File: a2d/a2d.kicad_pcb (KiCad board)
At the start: 4 copper layers, 70 x 65.8 mm, 76 parts, among them CN1 BM04B-SRSS-TB(LF)(SN), CN2 BM04B-SRSS-TB(LF)(SN), J1 Conn_02x04_Odd_Even, U1 B3B-XH-A(LF)(SN), U10 B3B-XH-A(LF)(SN), U2 2060-453/998-404, U3 ADM7150ARDZ-5.0, U4 ADS1115IDGSR, U5 2060-453/998-404, U6 B3B-XH-A(LF)(SN), U7 2060-453/998-404, U8 B3B-XH-A(LF)(SN), U9 2060-453/998-404

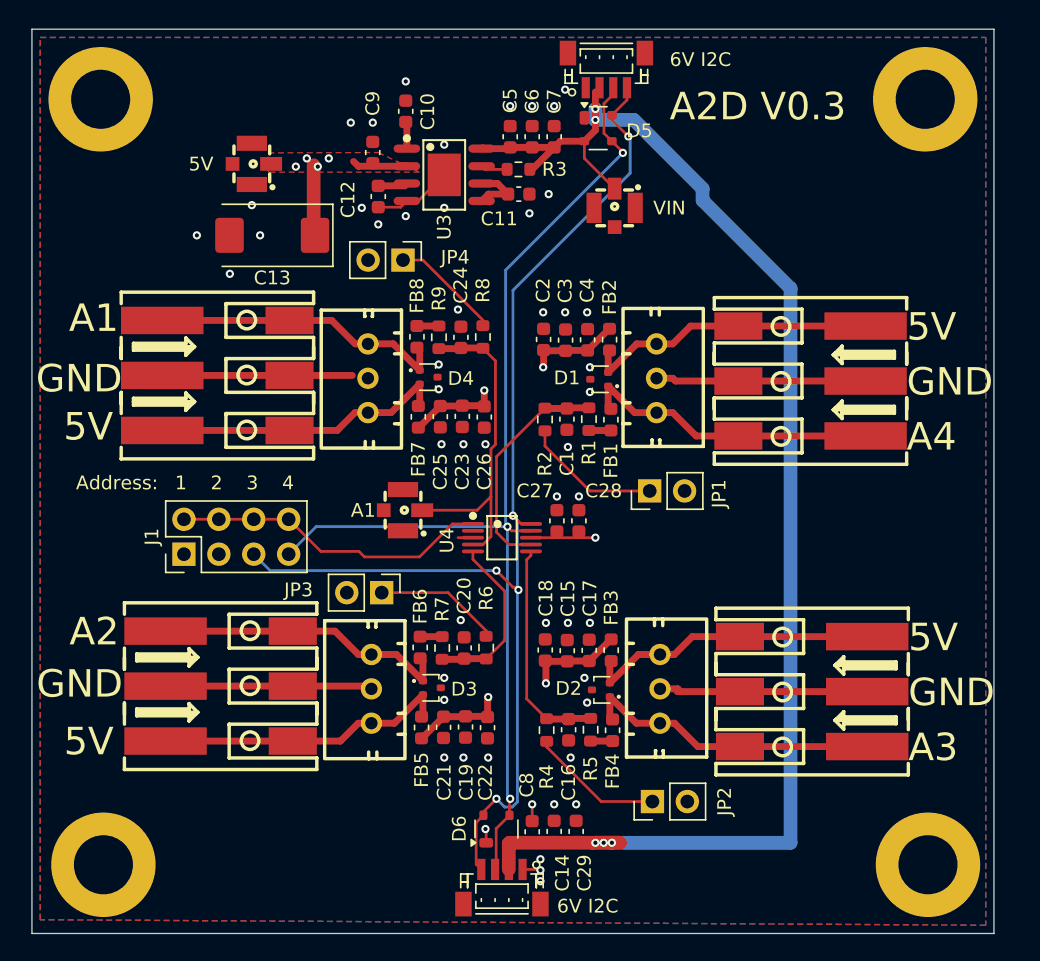
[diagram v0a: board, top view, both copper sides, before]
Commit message: a2d v0.4
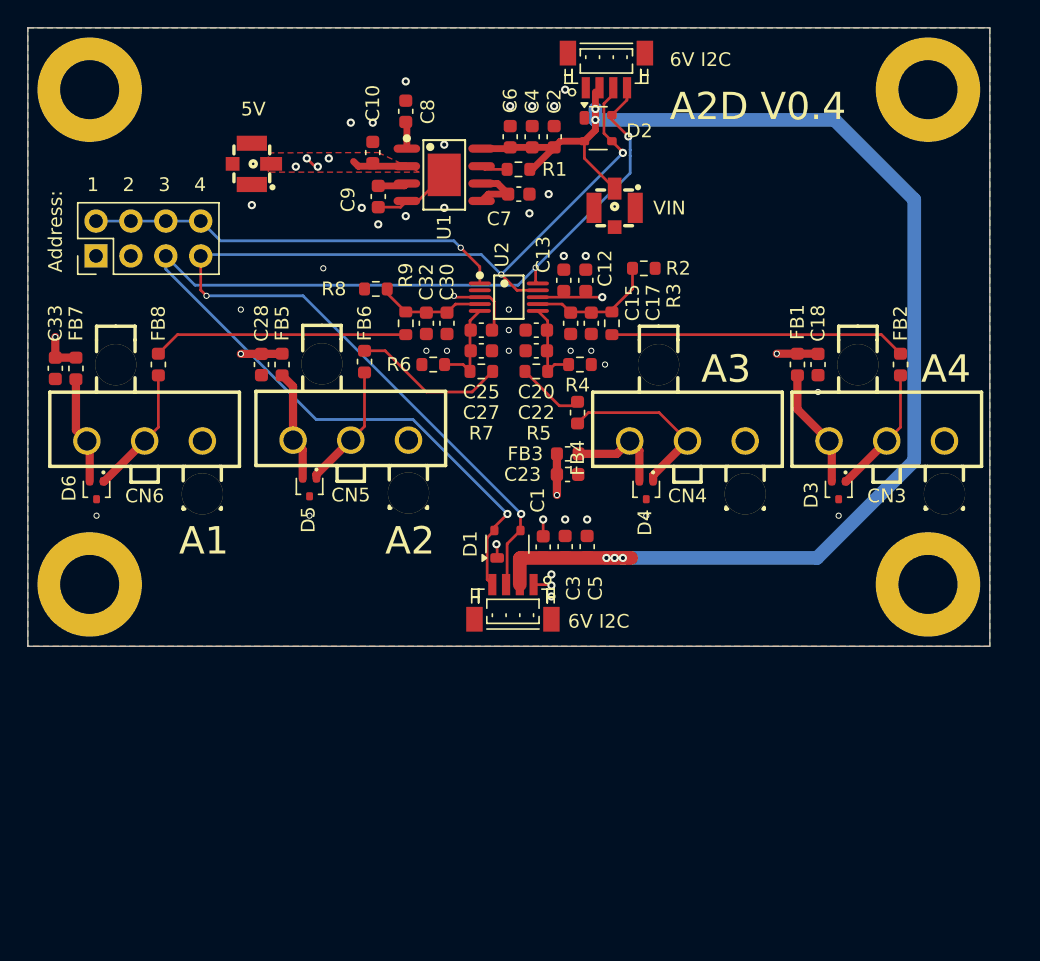
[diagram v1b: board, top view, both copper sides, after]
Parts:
- removed the C13 at (33.3, 30.6)
- removed the C15 at (54.8, 60.8)
- removed C19: 10uF, Capacitor_SMD:C_0603_1608Metric
- removed C21: 1uF, Capacitor_SMD:C_0603_1608Metric
- removed the C23 at (47.1, 43.8)
- removed the C25 at (45.5, 43.8)
- removed the C3 at (54.6, 38.2)
- removed the C4 at (56.2, 38.2)
- removed JP1, JP2, JP3, JP4: Jumper_2_Small_Open, Connector_PinHeader_2.54mm:PinHeader_1x02_P2.54mm_Vertical
- removed RF3: 73412-0110, easyeda2kicad:ANT-SMD_73412-0110
- removed the U1 at (61.2, 41.0)
- removed U10, U6, U8: B3B-XH-A(LF)(SN), easyeda2kicad:CONN-TH_3P-P2.50_A2501WV2-3P
- removed the U2 at (71.8, 41.2)
- removed U5, U7, U9: 2060-453/998-404, easyeda2kicad:CONN-SMD_2060-453
- added C22: 3.3uF, Capacitor_SMD:C_0603_1608Metric, F.Cu at (52.5, 39.0)
- added C27: 3.3uF, Capacitor_SMD:C_0603_1608Metric, F.Cu at (48.5, 39.0)
- added C32: 3.3uF, Capacitor_SMD:C_0603_1608Metric, F.Cu at (44.5, 37.0)
- added CN3: 39302030, easyeda2kicad:CONN-TH_3P-P4.20_39302030, F.Cu at (78.0, 45.6)
- added CN4: 39302030, easyeda2kicad:CONN-TH_3P-P4.20_39302030, F.Cu at (63.5, 45.6)
- added CN5: 39302030, easyeda2kicad:CONN-TH_3P-P4.20_39302030, F.Cu at (39.0, 45.5)
- added CN6: 39302030, easyeda2kicad:CONN-TH_3P-P4.20_39302030, F.Cu at (24.0, 45.6)
- C17: value 1uF -> 3.3uF
- moved C33 31.4 mm to (17.5, 40.3)
- moved C28 31.1 mm to (32.5, 40.0)
- moved C20 29.2 mm to (52.5, 37.5), turned to 0 degrees
- moved FB5 28.3 mm to (34.0, 40.0), turned to 90 degrees
- moved R4 26.7 mm to (55.7, 40.0), turned to 180 degrees
- moved R5 26.4 mm to (52.5, 40.5), turned to 180 degrees
- moved D6 25.5 mm to (20.5, 49.1), turned to -90 degrees
- moved FB7 25.2 mm to (19.0, 40.3), turned to 90 degrees
- moved C17 23.8 mm to (56.5, 37.0)
- moved FB4 23.3 mm to (55.5, 43.5), turned to 90 degrees
- moved C25 23.2 mm to (48.5, 37.5), turned to 180 degrees
- moved J1 22.6 mm to (20.5, 32.1)
- moved FB2 21.4 mm to (79.0, 40.0), turned to 90 degrees
- moved FB6 21.2 mm to (40.0, 39.8)
- moved R6 21.0 mm to (45.0, 40.0), turned to 0 degrees
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- renumbered C8 to C1, C9 to C10, C28 to C12, C27 to C13, C1 to C15, C2 to C18, C7 to C2, C16 to C20, C18 to C23, C20 to C25, C22 to C28, C14 to C3, C24 to C30, C26 to C33, C6 to C4, C29 to C5, C5 to C6, C11 to C7, C10 to C8, C12 to C9, CN2 to CN1, CN1 to CN2, D6 to D1, D5 to D2, D1 to D3, D2 to D4, D3 to D5, D4 to D6, FB2 to FB1, FB1 to FB2, R3 to R1, R1 to R3, U3 to U1, U4 to U2
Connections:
- C17 pad 1: +5V -> GND
- C17 pad 2: GND -> /A4
- R2 pad 1: Net-(JP1-A) -> GND
- R4 pad 1: Net-(JP2-A) -> GND
- R6 pad 1: Net-(JP3-A) -> GND
- R8 pad 1: Net-(JP4-A) -> GND
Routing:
- net GND: track 69.2 -> 13.8 mm, vias 51 -> 40
- net +5V: track 41.3 -> 21.2 mm
- net Net-(FB2-Pad2): track 1.60 -> 21.6 mm
- net Net-(FB8-Pad2): track 1.60 -> 18.6 mm
- net /A1: track 24.3 -> 7.90 mm
- net Net-(D4-K2): track 21.6 -> 7.34 mm
- net Net-(D6-K2): track 21.6 -> 7.84 mm
- net Net-(D5-K2): track 21.6 -> 8.12 mm
- net Net-(D3-K2): track 21.6 -> 8.75 mm
- net Net-(D5-K1): track 22.0 -> 9.16 mm
- net Net-(D6-K1): track 22.0 -> 9.41 mm
- net Net-(D3-K1): track 22.0 -> 9.41 mm
- net Net-(JP1-A): track 10.5 -> 0.00 mm
- net Net-(JP2-A): track 9.75 -> 0.00 mm
- net /A3: track 16.0 -> 6.43 mm
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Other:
- board size 70 x 65.8 mm -> 70 x 45 mm
- board text added: "A2D V0.4"
- board text removed: "A2D V0.3"
- board text removed: "GND"
